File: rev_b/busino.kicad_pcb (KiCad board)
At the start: 2 copper layers, 100 x 100 mm, 62 parts, among them J1 TERMINATE_JUMPER, J2 LED_JUMPER, SW1 2_LEAD_PUSH_BUTTON, U1 LM2940CT-5.0, U2 MCP2562, U3 LM1117T-3.3, U4 74x06, U5 ATMEGA324_DIP40, X1 16MHz, X2 OSHW_LOGO

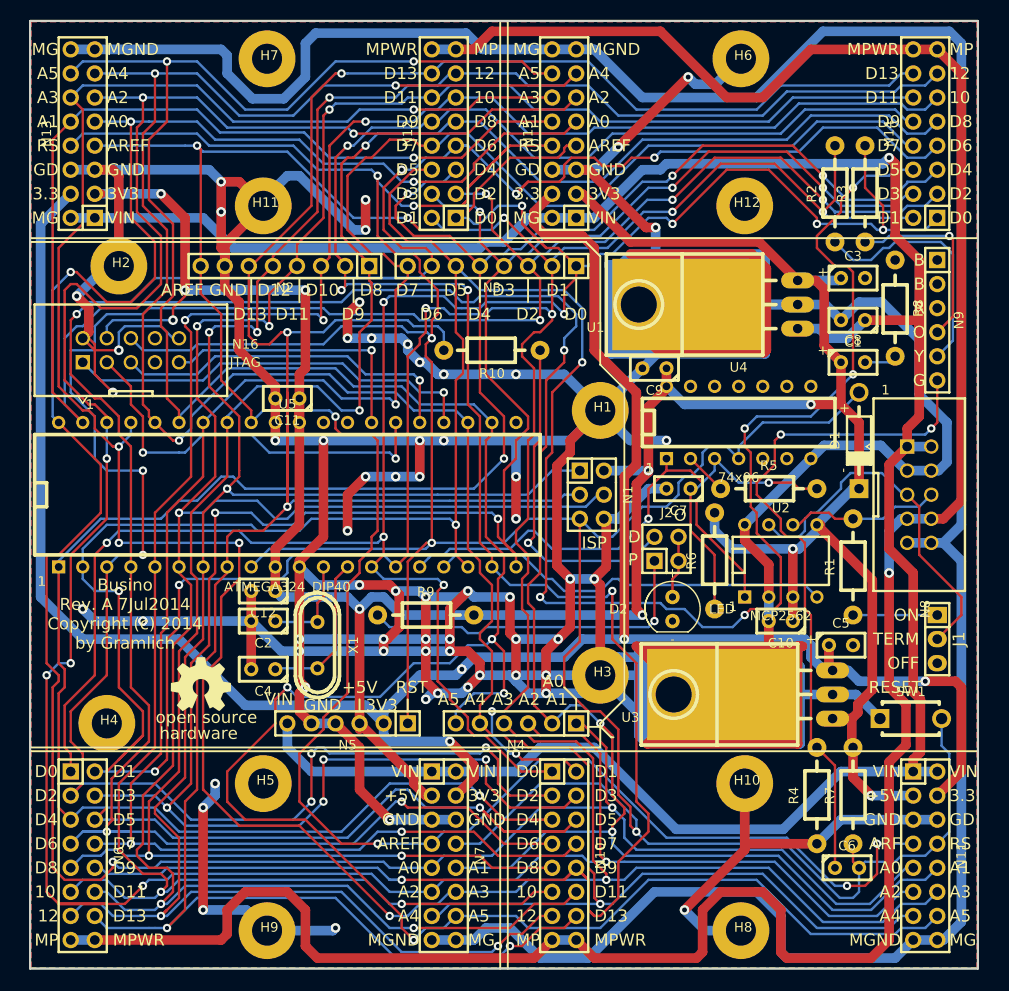
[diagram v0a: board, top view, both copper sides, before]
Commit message: Add in some derived files.
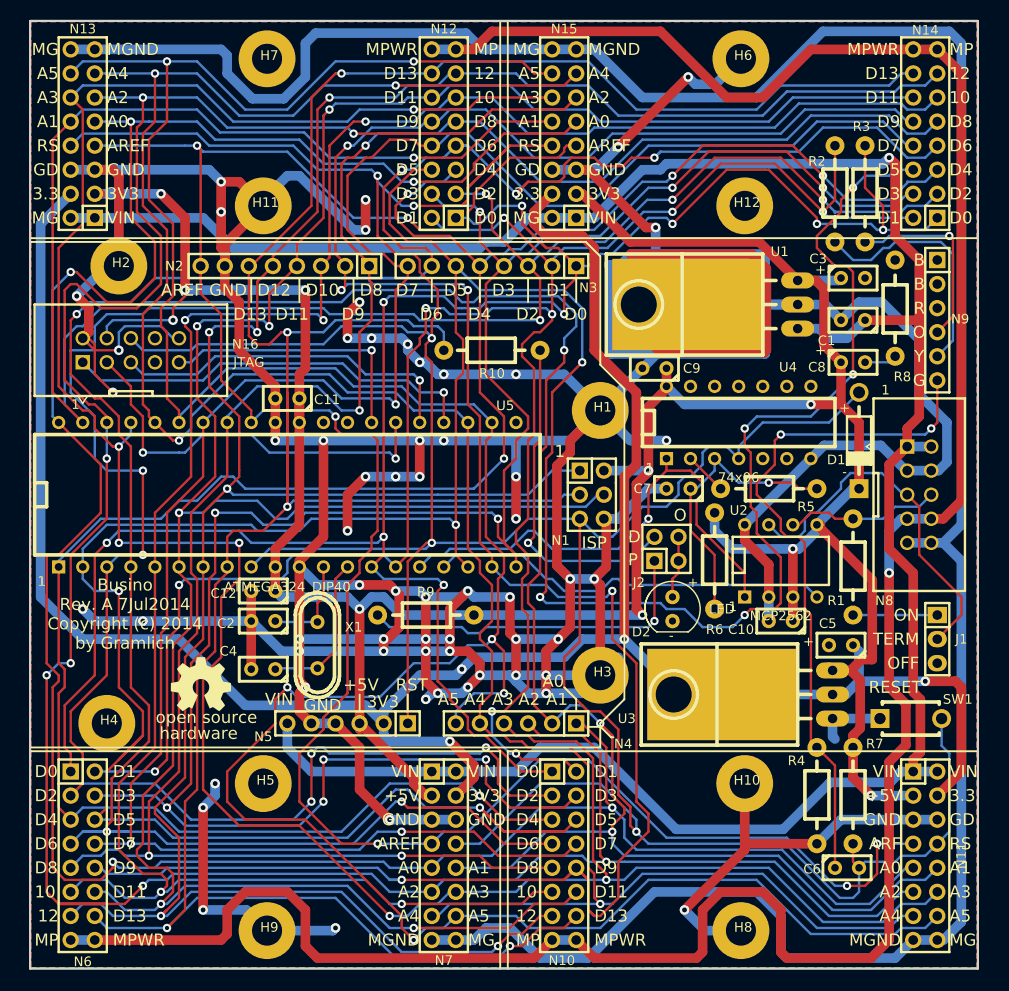
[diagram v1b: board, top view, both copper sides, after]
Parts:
- D1: value SCHOTTKY_DIODE_VERT -> SD101C-TR
- R10, R9: value R_VERT -> 470
- U3: value LM1117T-3.3 -> LM1117
- turned C5 to 180 degrees
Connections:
- U3 pad 1: VCC -> GND
- U3 pad 2: GND -> +3.3V
- U3 pad 3: +3.3V -> VCC
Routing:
- net GND: track 943.1 -> 816.6 mm
- net VCC: track 320.5 -> 324.5 mm
- net +3.3V: track 241.1 -> 243.1 mm
